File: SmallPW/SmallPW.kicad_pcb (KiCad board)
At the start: 2 copper layers, 28.3 x 11 mm, 22 parts, among them J1 Conn_01x02_Male, J2 Conn_01x02_Female, J3 Conn_01x02_Female, J4 Conn_01x02_Female, J5 Conn_01x02_Female, Q1 MTP4835I3, Q2 BSS138, Q3 MTP4835I3, SW1 SW_SPST

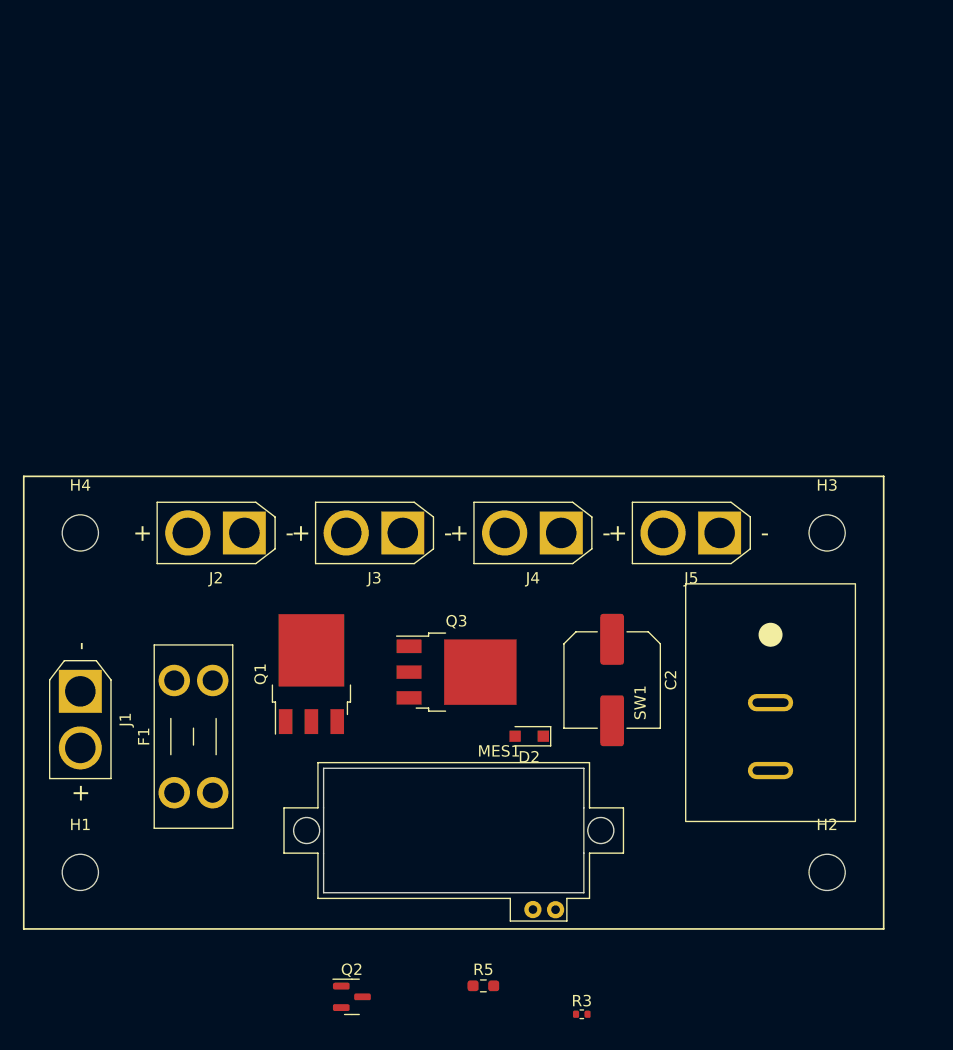
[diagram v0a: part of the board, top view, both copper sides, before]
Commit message: LargeMDほぼ完成
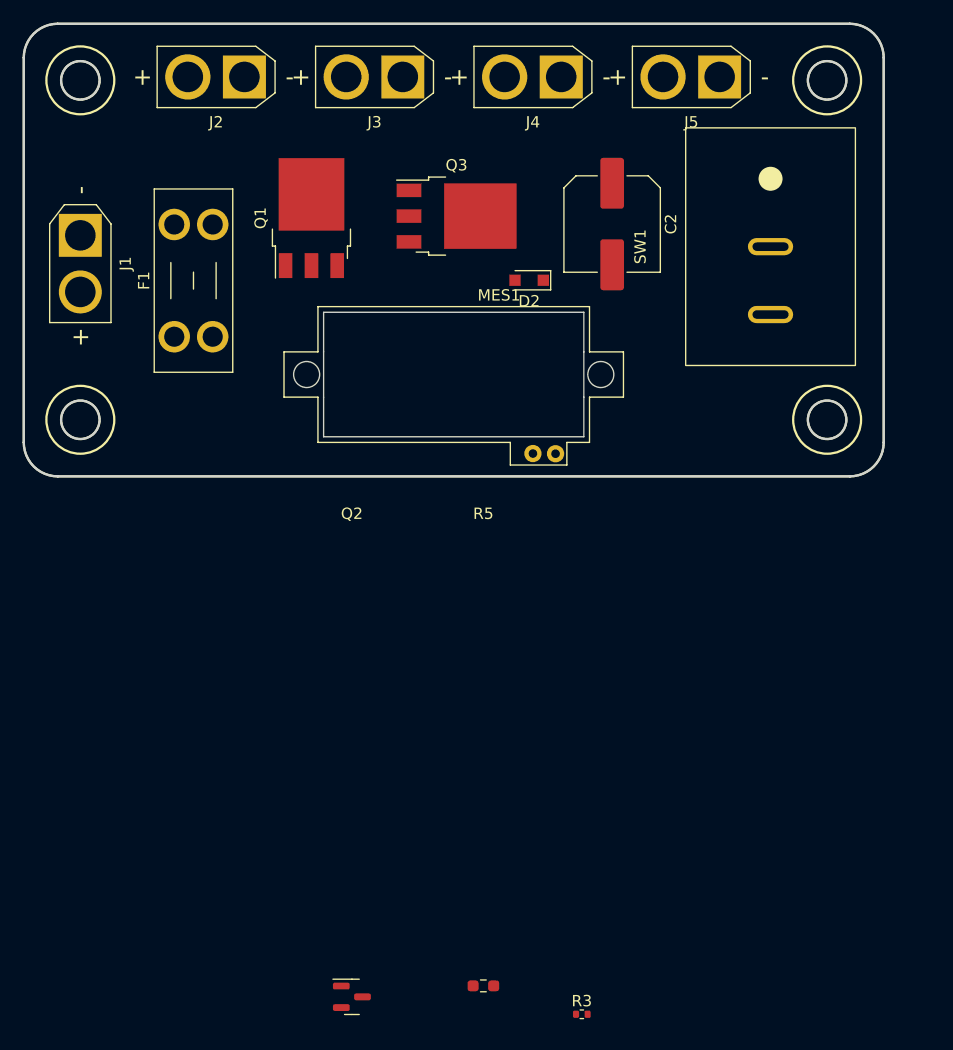
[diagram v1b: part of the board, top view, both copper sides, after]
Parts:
- removed H1, H2, H3, H4: MountingHole, MountingHole:MountingHole_3.2mm_M3
- moved C2 40.3 mm to (52.0, -22.3)
- moved D2 40.3 mm to (44.7, -17.3)
- moved F1 40.3 mm to (13.3, -12.3)
- moved J1 40.3 mm to (5.00, -21.3)
- moved J2 40.3 mm to (19.5, -35.3)
- moved J3 40.3 mm to (33.5, -35.3)
- moved J4 40.3 mm to (47.5, -35.3)
- moved J5 40.3 mm to (61.5, -35.3)
- moved MES1 40.3 mm to (38.0, -9.00)
- moved Q1 40.3 mm to (25.4, -22.8)
- moved Q3 40.3 mm to (38.2, -23.0)
- moved SW1 40.3 mm to (66.0, -20.3)
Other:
- board size 28.3 x 11 mm -> 76 x 40 mm

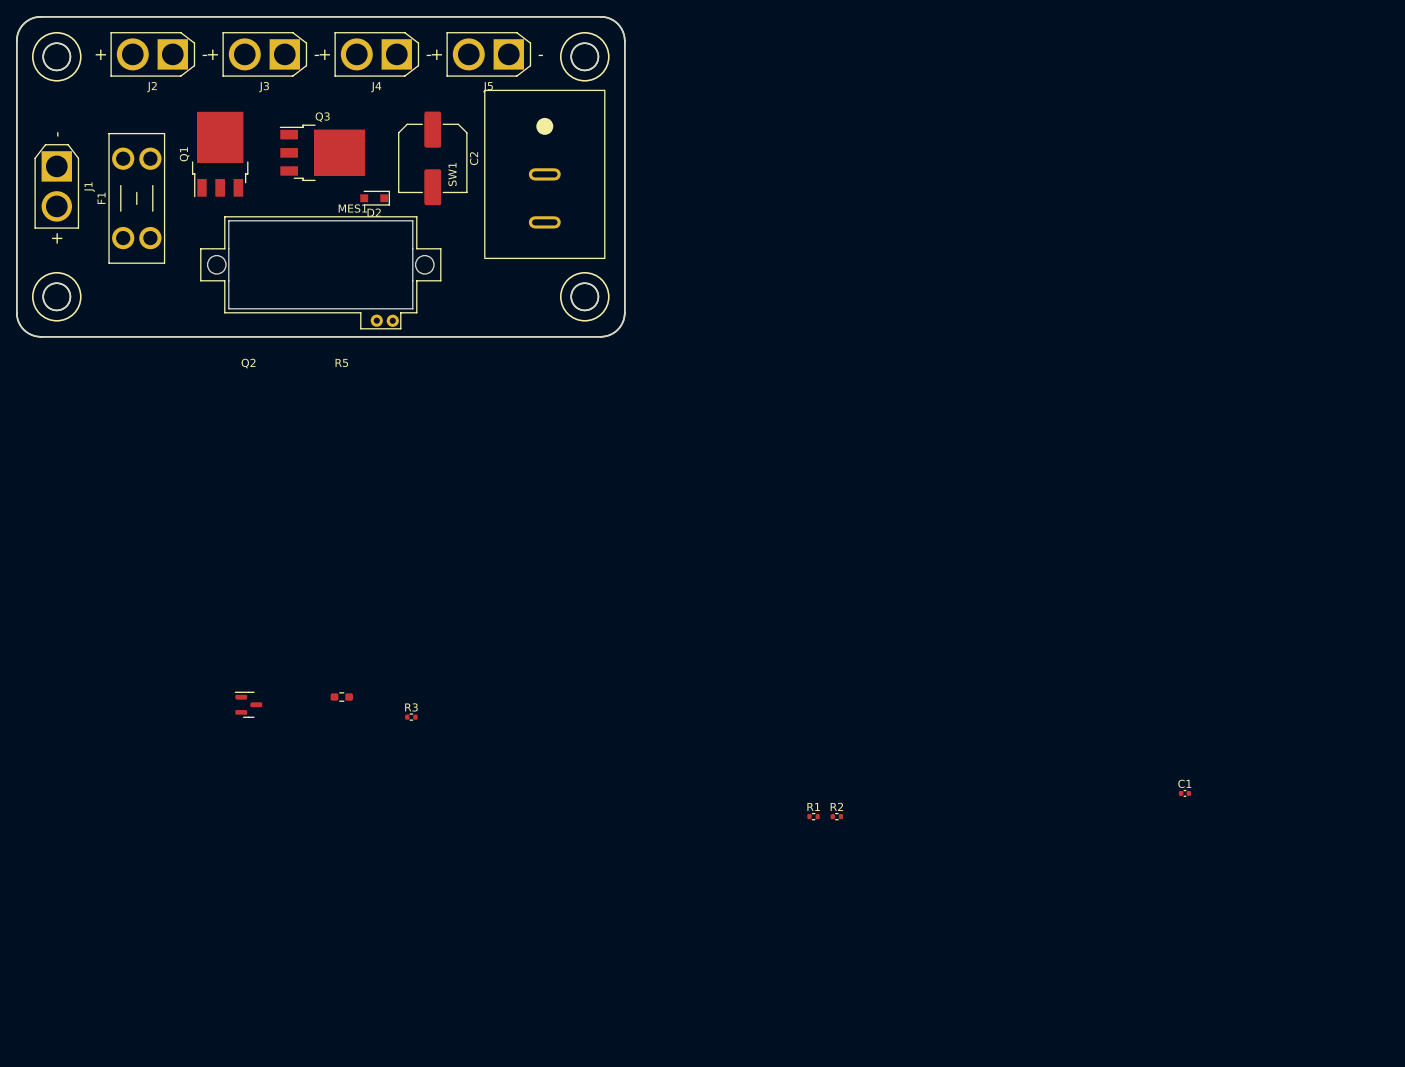
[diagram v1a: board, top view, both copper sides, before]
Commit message: SmallMDほぼ完成
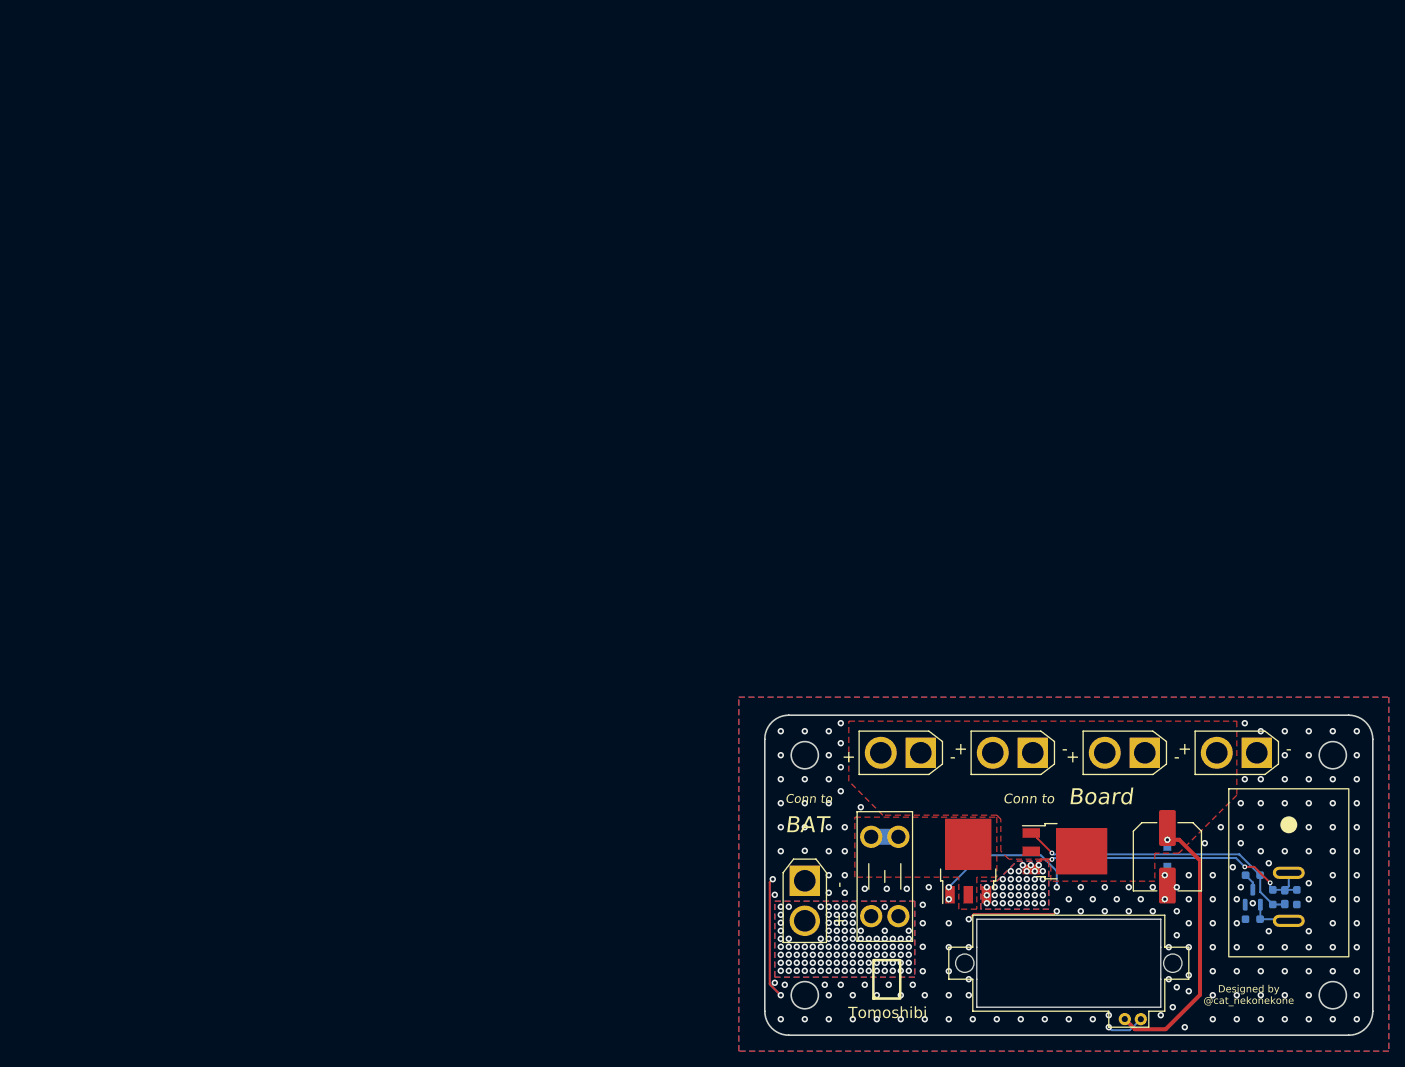
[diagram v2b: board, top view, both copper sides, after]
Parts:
- C1: footprint Capacitor_SMD:C_0402_1005Metric -> Capacitor_SMD:C_0603_1608Metric_Pad1.08x0.95mm_HandSolder; moved to B.Cu
- D2, Q2, R5: moved to B.Cu
- R1, R2, R3: footprint Resistor_SMD:R_0402_1005Metric -> Resistor_SMD:R_0603_1608Metric_Pad0.98x0.95mm_HandSolder; moved to B.Cu
- moved J1 129.3 mm to (98.5, 68.0)
- moved D2 128.9 mm to (143.8, 65.0), turned to -90 degrees
- moved Q1 128.7 mm to (118.9, 65.5)
- moved J2 127.9 mm to (113.0, 52.0)
- moved J3 127.9 mm to (127.0, 52.0)
- moved J4 127.9 mm to (141.0, 52.0)
- moved J5 127.9 mm to (155.0, 52.0)
- moved MES1 127.9 mm to (131.5, 78.3)
- moved Q2 127.8 mm to (154.5, 70.0), turned to 90 degrees
- moved SW1 127.6 mm to (159.0, 67.0)
- moved Q3 127.4 mm to (131.0, 64.3)
- moved C2 126.7 mm to (143.8, 65.0)
- moved F1 126.2 mm to (106.8, 72.4)
- moved R5 117.2 mm to (154.5, 72.8), turned to 180 degrees
- moved R3 107.0 mm to (154.5, 67.3), turned to 180 degrees
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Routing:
- net GND: track 0.00 -> 76.0 mm, vias 0 -> 189
- net /S-S: track 0.00 -> 38.2 mm, vias 0 -> 41
- net 主電源スイッチ: track 0.00 -> 36.4 mm, vias 0 -> 1
- net VDD: track 0.00 -> 34.5 mm, vias 0 -> 1
- net Net-(Q2-Pad1): track 0.00 -> 5.50 mm
- net Net-(F1-Pad2): track 0.00 -> 3.40 mm
- net Net-(Q2-Pad3): track 0.00 -> 2.19 mm
- net /12VBAT: vias 0 -> 108
- added copper zone on B.Cu, net /12VBAT
- added copper zone on F.Cu, net /12VBAT
- added copper zone on B.Cu, net /S-S
- added copper zone on F.Cu, net /S-S
- added copper zone on B.Cu, net GND
- added copper zone on F.Cu, net GND
- added copper zone on F.Cu, net Net-(F1-Pad2)
- added copper zone on F.Cu, net VDD
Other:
- board text added: "BAT"
- board text added: "Board"
- board text added: "Conn to"
- board text added: "Designed by @cat_nekonekone"
- board text added: "Tomoshibi"
- board text added: "燈"
